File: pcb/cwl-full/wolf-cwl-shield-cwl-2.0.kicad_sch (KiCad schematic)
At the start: 30 parts, among them J1 UEXT, J2 OpenTherm, J3 OLED_1.3, J4 OLED_0.96, Q1 BC858A, SW1 EC12E24204A9, U1 PC817, U2 PC817

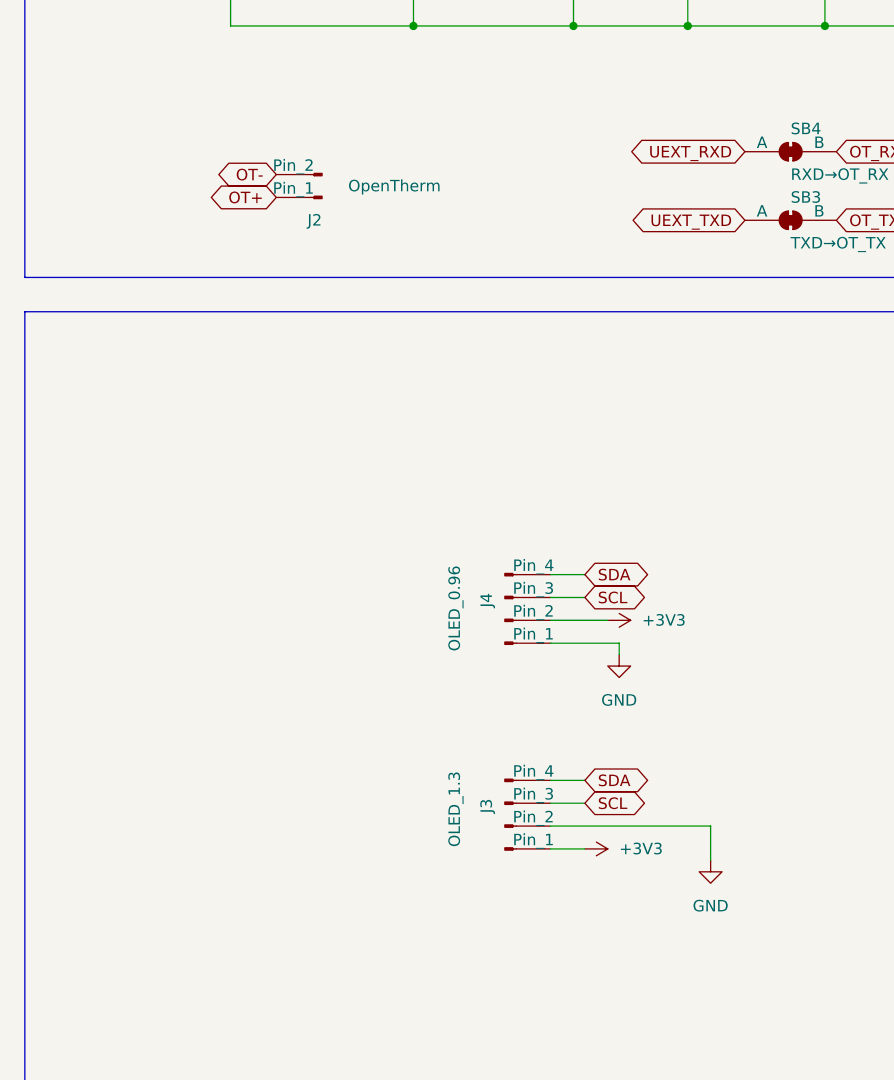
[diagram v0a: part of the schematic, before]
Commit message: new pcb
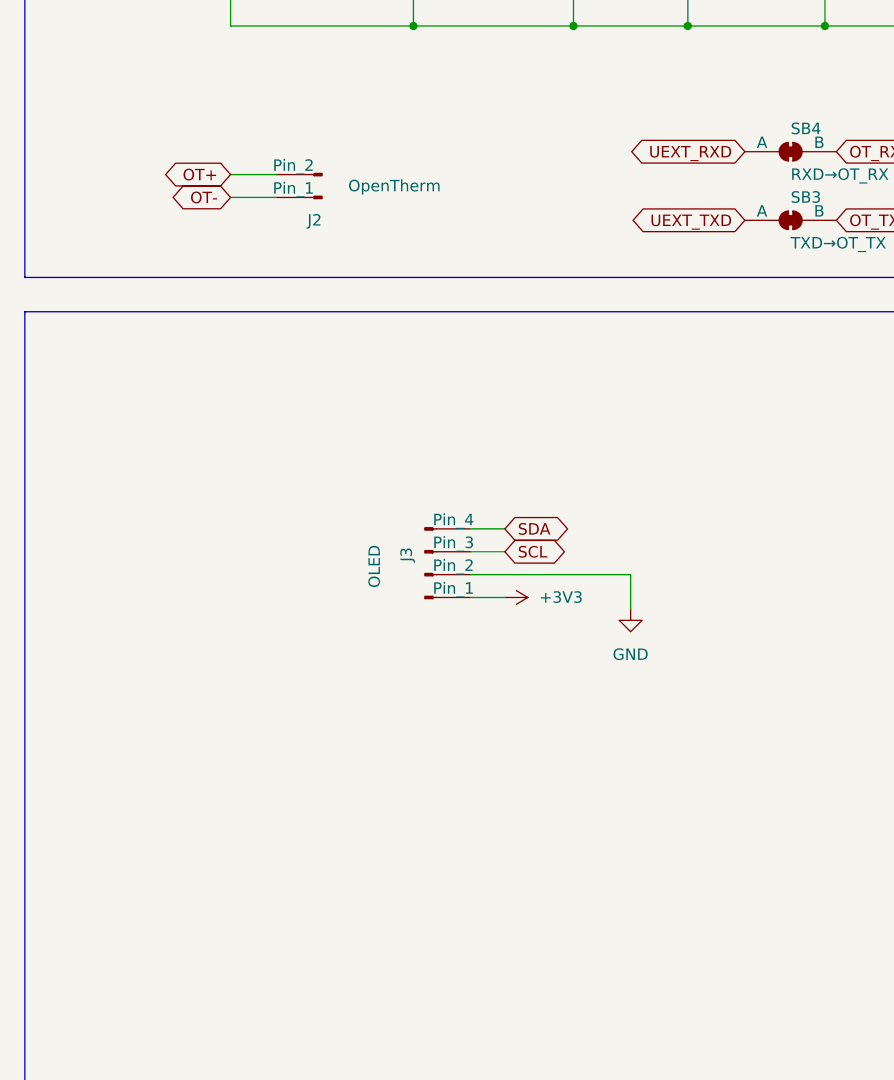
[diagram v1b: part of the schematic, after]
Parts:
- removed J4: OLED_0.96, SSD1306:128x64OLED-MountingHoles, symbol Connector:Conn_01x04_Pin
- D5, D6, D7: footprint Diode_SMD:D_SOD-323 -> Diode_SMD:D_SOD-123
- J3: value OLED_1.3 -> OLED; footprint SSD1306:128x64OLED-MountingHoles-Large -> SSD1306:128x64OLED-MountingHoles-Combined
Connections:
- net OT+: now also J2.2 (Pin_2); no longer J2.1 (Pin_1)
- net OT-: now also J2.1 (Pin_1); no longer J2.2 (Pin_2)
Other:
- moved on the sheet: J3
